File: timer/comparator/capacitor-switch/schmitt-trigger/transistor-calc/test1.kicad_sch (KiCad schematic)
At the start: 10 parts, among them Q1 NPN, Q2 NPN

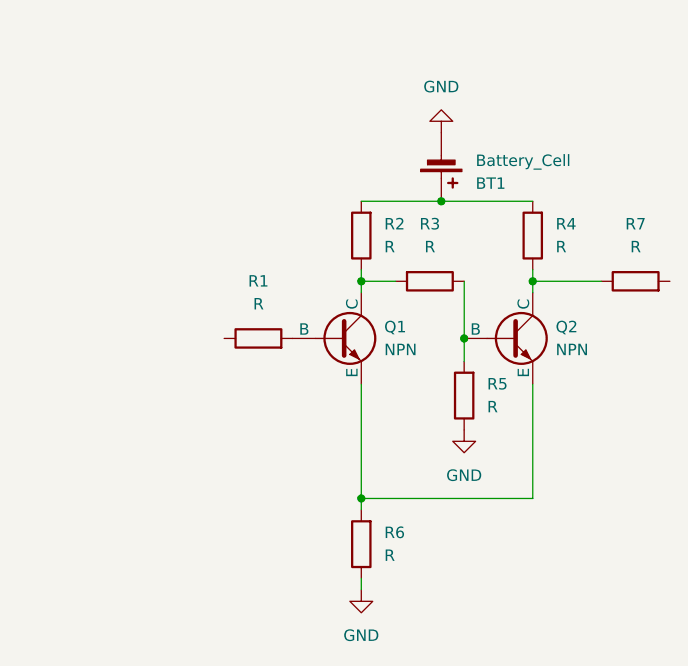
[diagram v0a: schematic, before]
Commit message: add/fix
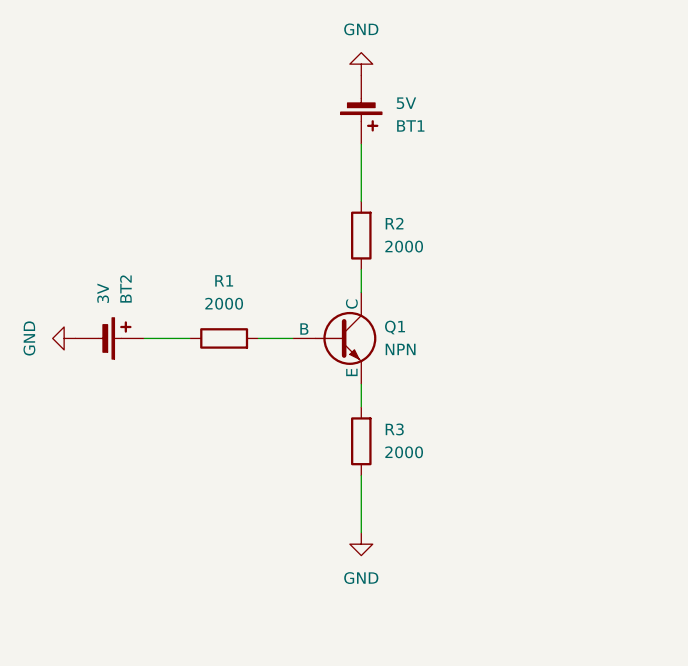
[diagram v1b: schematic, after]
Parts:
- removed Q2: NPN, symbol Simulation_SPICE:NPN
- removed R4, R5, R6, R7: R, symbol Device:R
- added BT2: 3V, symbol Device:Battery_Cell
- BT1: value Battery_Cell -> 5V
- R1, R2, R3: value R -> 2000
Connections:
- net GND: now also R3.1, BT2.2 (-)
- net at Q1.3 (E): now also R3.2
- net at Q1.1 (C), R2.1: no longer R3.2
- net at R1.1: now also BT2.1 (+)
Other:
- moved on the sheet: BT1, R1
